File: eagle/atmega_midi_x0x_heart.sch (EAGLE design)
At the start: 32 parts, among them IC1 TL072P, J11_VCF_CUTOFF 22-23-2021, U1 ATMEGA328P_PDIP

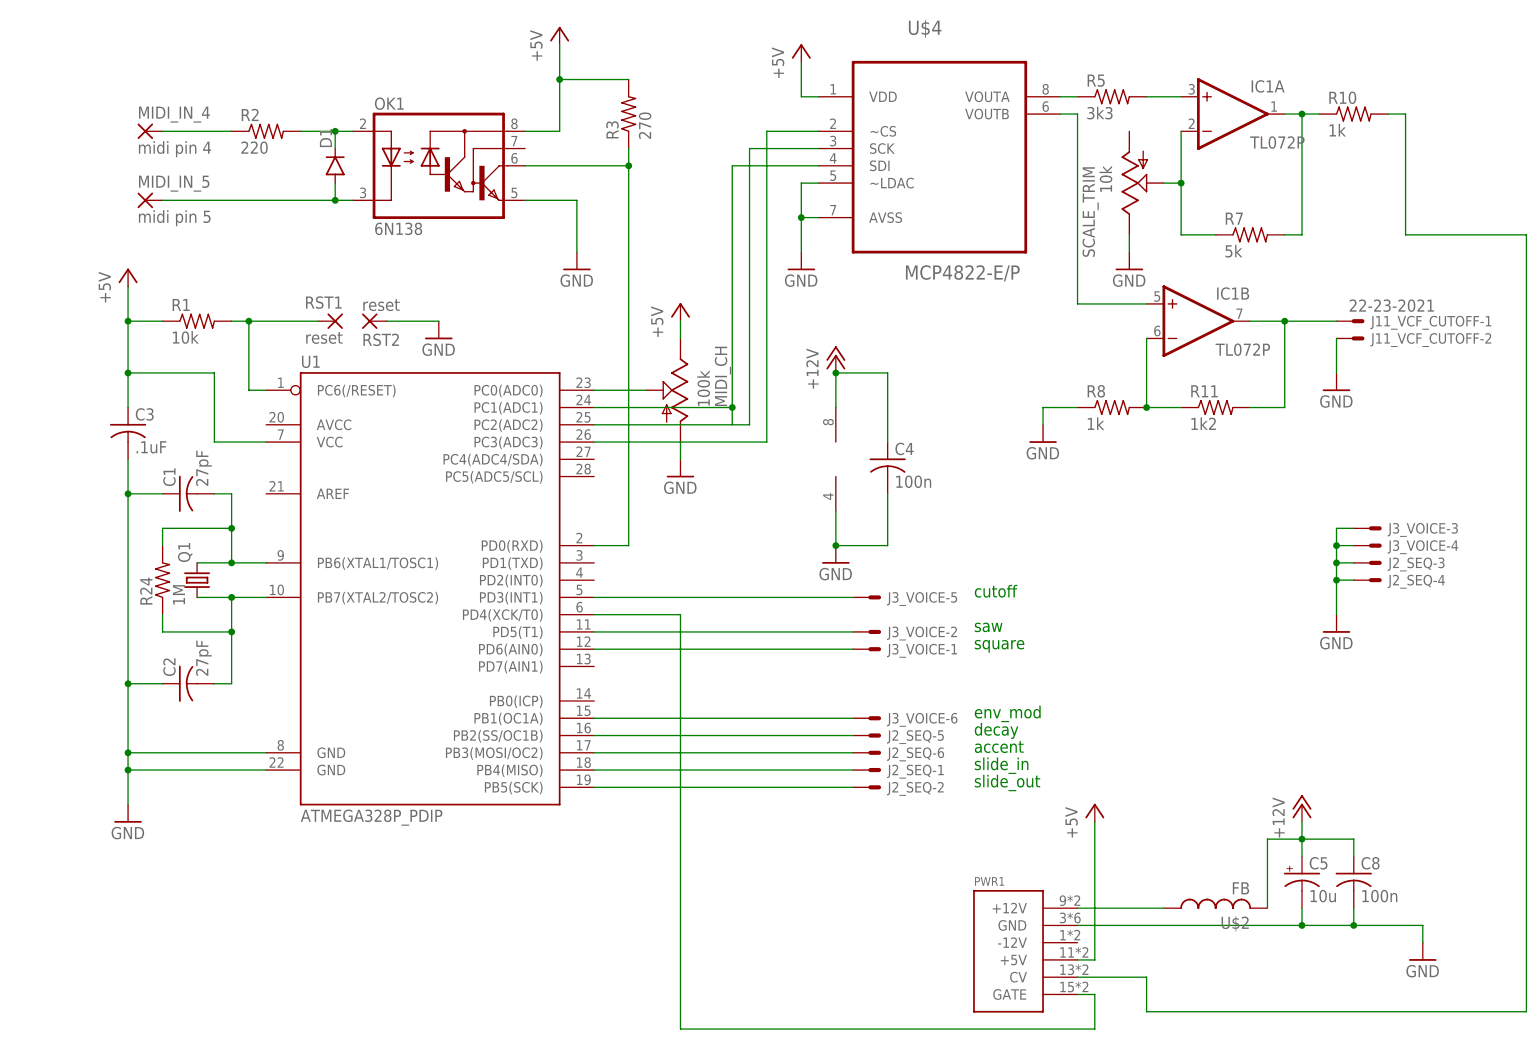
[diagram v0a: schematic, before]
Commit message: niced up schemo
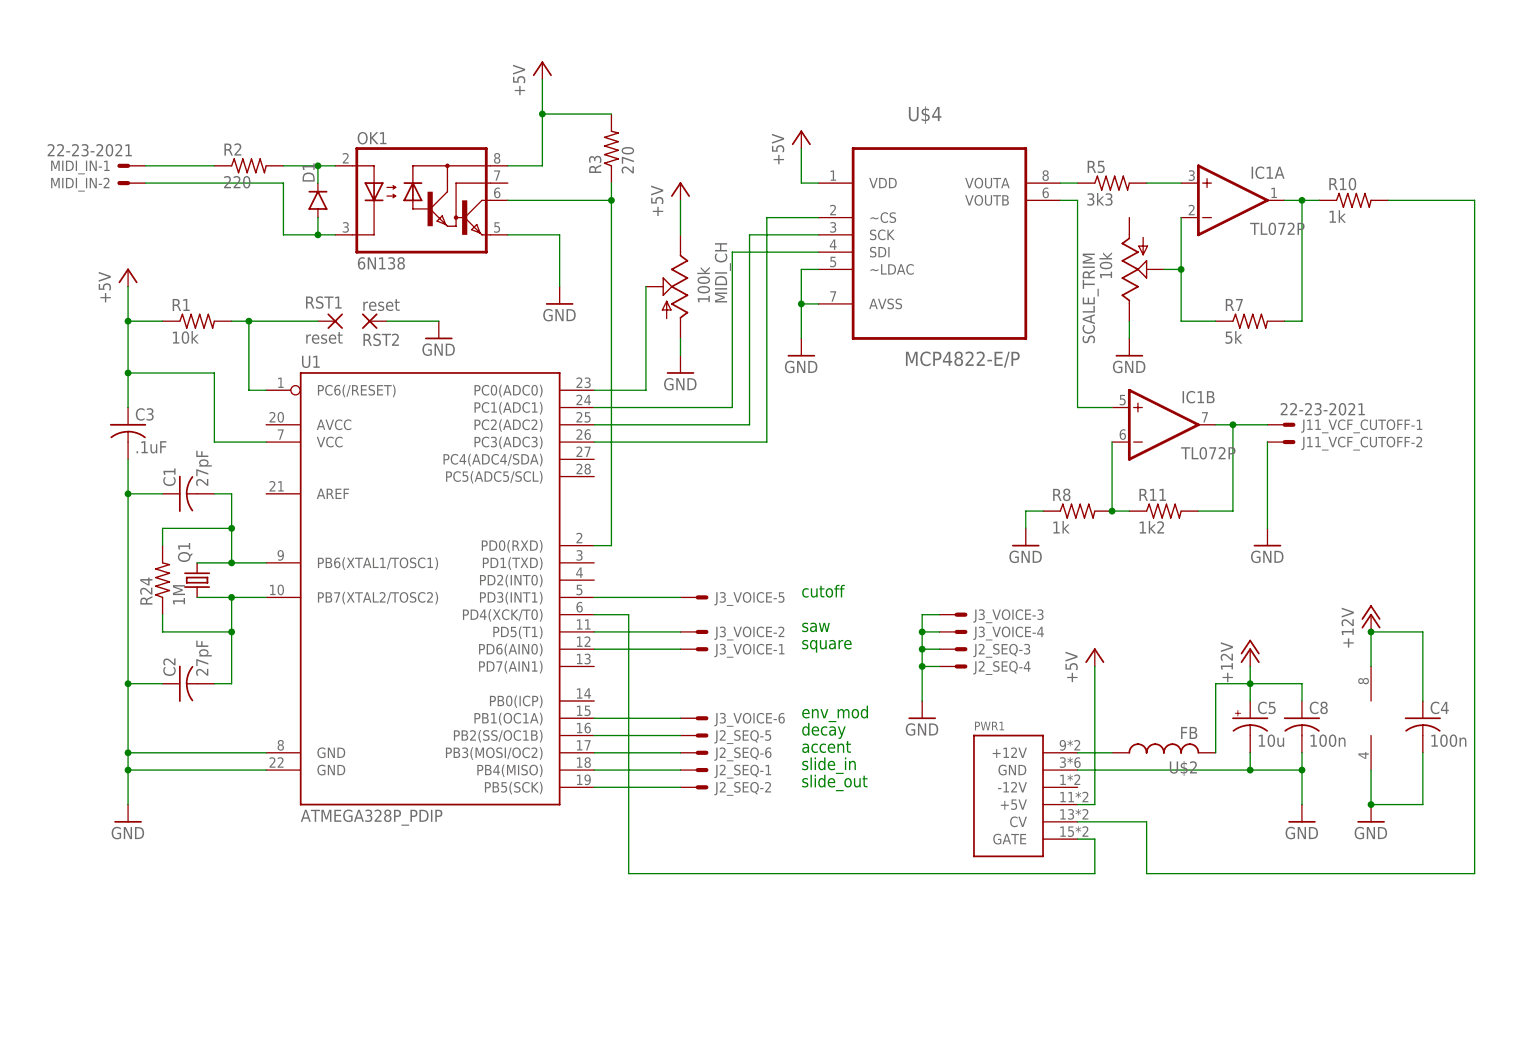
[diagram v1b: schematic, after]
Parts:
- removed MIDI_IN_4: midi pin 4, wirepad:2,54/0,9
- removed MIDI_IN_5: midi pin 5, wirepad:2,54/0,9
- added MIDI_IN: 22-23-2021, con-molex:22-23-2021
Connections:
- net N$3: now also MIDI_IN-2.S; no longer MIDI_IN_5.P
- net N$8: now also MIDI_IN-1.S; no longer MIDI_IN_4.P
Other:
- moved on the sheet: C4, C5, C8, D1, IC1A, IC1B, J11_VCF_CUTOFF-1, J11_VCF_CUTOFF-2, J2_SEQ-1, J2_SEQ-2, J2_SEQ-3, J2_SEQ-4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
